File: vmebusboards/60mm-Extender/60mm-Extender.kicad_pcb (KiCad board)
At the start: 2 copper layers, 2 parts, among them U1 VME64-P1-3R, U2 VME64-P1-3R

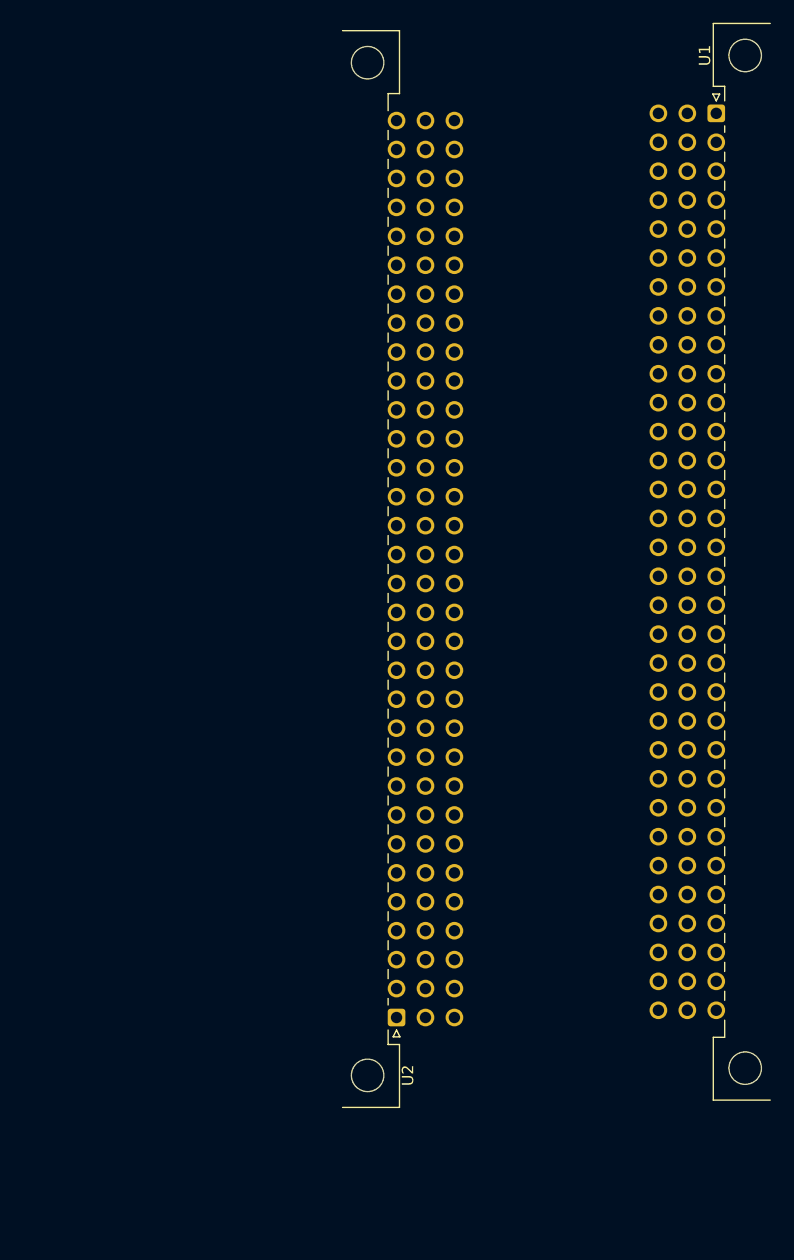
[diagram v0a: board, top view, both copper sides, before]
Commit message: Updated
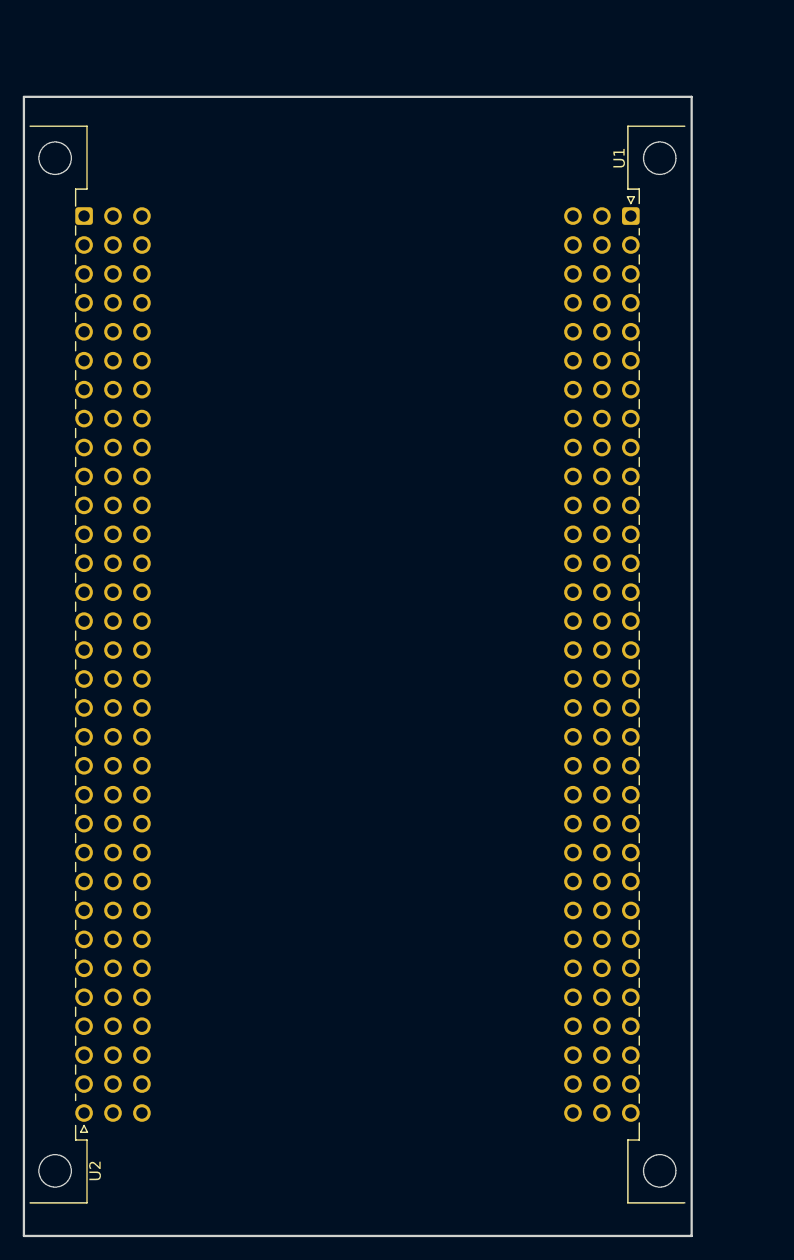
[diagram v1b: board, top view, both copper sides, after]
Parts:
- U2: footprint Connector_DIN:DIN41612_R_3x32_Female_Horizontal_THT -> Computie_Connectors:DIN41612_R_3x32_Reverse_Female_Horizontal_THT
- moved U2 28.7 mm to (49.5, 114.3)
- moved U1 11.7 mm to (97.5, 35.6)
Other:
- board outline added: 58.6 x 100 mm
